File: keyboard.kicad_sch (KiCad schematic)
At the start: 136 parts, among them J1 Conn_01x06_Socket, J2 Conn_01x02_Socket, J3 Conn_01x02_Socket, J4 Conn_01x06_Socket, SW1 SW_Push, SW10 SW_Push, SW11 SW_Push, SW12 SW_Push, SW13 SW_Push, SW14 SW_Push, SW15 SW_Push, SW16 SW_Push, SW17 SW_Push, SW18 SW_Push, SW19 SW_Push, SW2 SW_Push, SW20 SW_Push, SW21 SW_Push, SW22 SW_Push, SW23 SW_Push, SW24 SW_Push, SW25 SW_Push, SW26 SW_Push, SW27 SW_Push, SW28 SW_Push, SW29 SW_Push, SW3 SW_Push, SW30 SW_Push, SW31 SW_Push, SW32 SW_Push, SW33 SW_Push, SW34 SW_Push, SW35 SW_Push, SW36 SW_Push, SW37 SW_Push, SW38 SW_Push, SW39 SW_Push, SW4 SW_Push, SW40 SW_Push, SW41 SW_Push, SW42 SW_Push, SW43 SW_Push, SW44 SW_Push, SW45 SW_Push, SW46 SW_Push, SW47 SW_Push, SW48 SW_Push, SW49 SW_Push, SW5 SW_Push, SW50 SW_Push, SW51 SW_Push, SW52 SW_Push, SW53 SW_Push, SW54 SW_Push, SW55 SW_Push, SW56 SW_Push, SW57 SW_Push, SW58 SW_Push, SW59 SW_Push, SW6 SW_Push, SW60 SW_Push, SW7 SW_Push, SW8 SW_Push, SW9 SW_Push, U1 rp2040-zero, U2 rp2040-zero

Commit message: 実は耐えてた
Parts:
- U1: footprint mcu:rp2040-zero-tht -> mcu:rp2040-zero-smd_reverse_flush_A
- U2: footprint mcu:rp2040-zero-tht -> mcu:rp2040-zero-smd_reverse_flush_B
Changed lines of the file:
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@@
 			)
 		)
-		(property "Footprint" "mcu:rp2040-zero-tht"
+		(property "Footprint" "mcu:rp2040-zero-smd_reverse_flush_A"
 			(at 88.9 48.26 0)
 			(effects
@@
 			)
 		)
-		(property "Footprint" "mcu:rp2040-zero-tht"
+		(property "Footprint" "mcu:rp2040-zero-smd_reverse_flush_B"
 			(at 223.52 48.26 0)
 			(effects

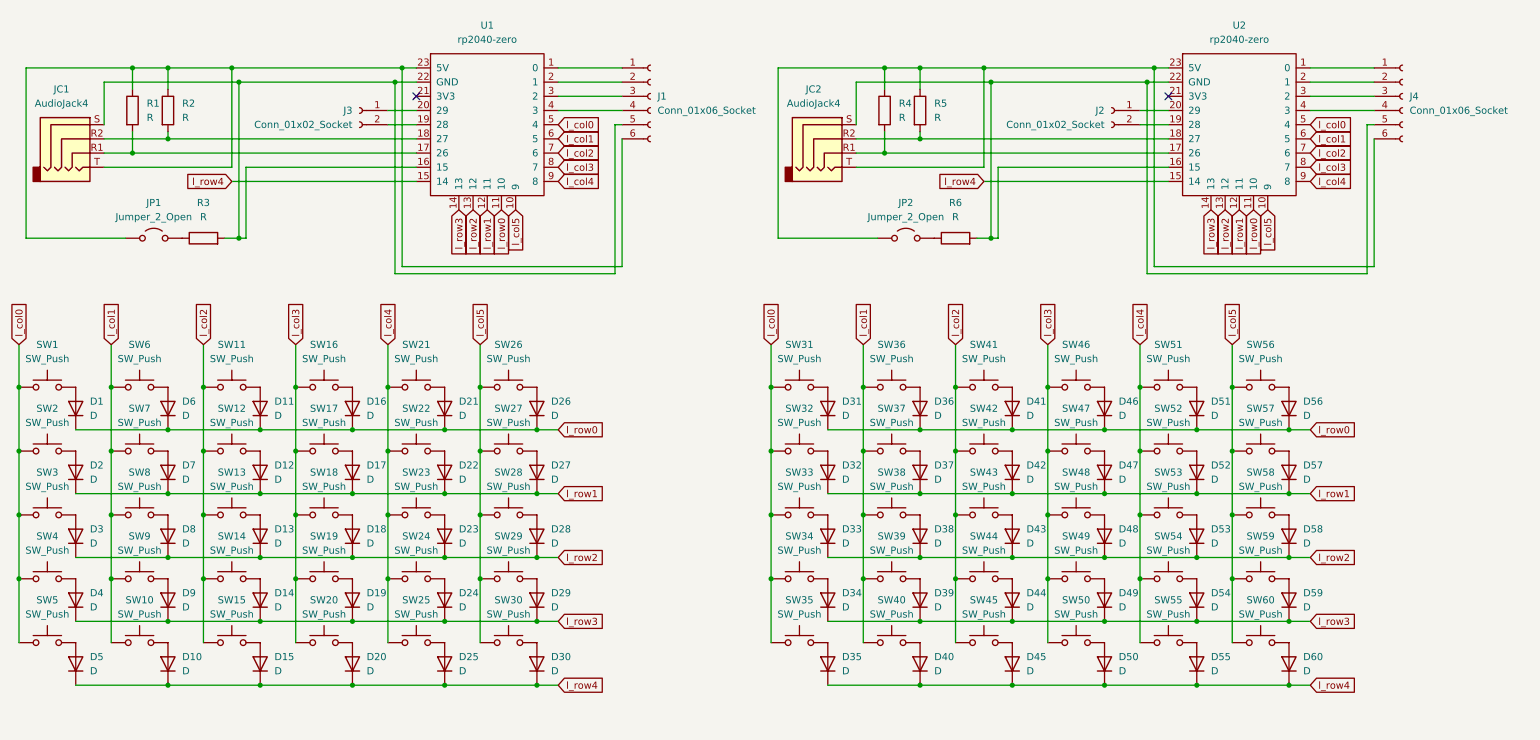
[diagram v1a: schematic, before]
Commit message: 抵抗の配置を直したのでcommit
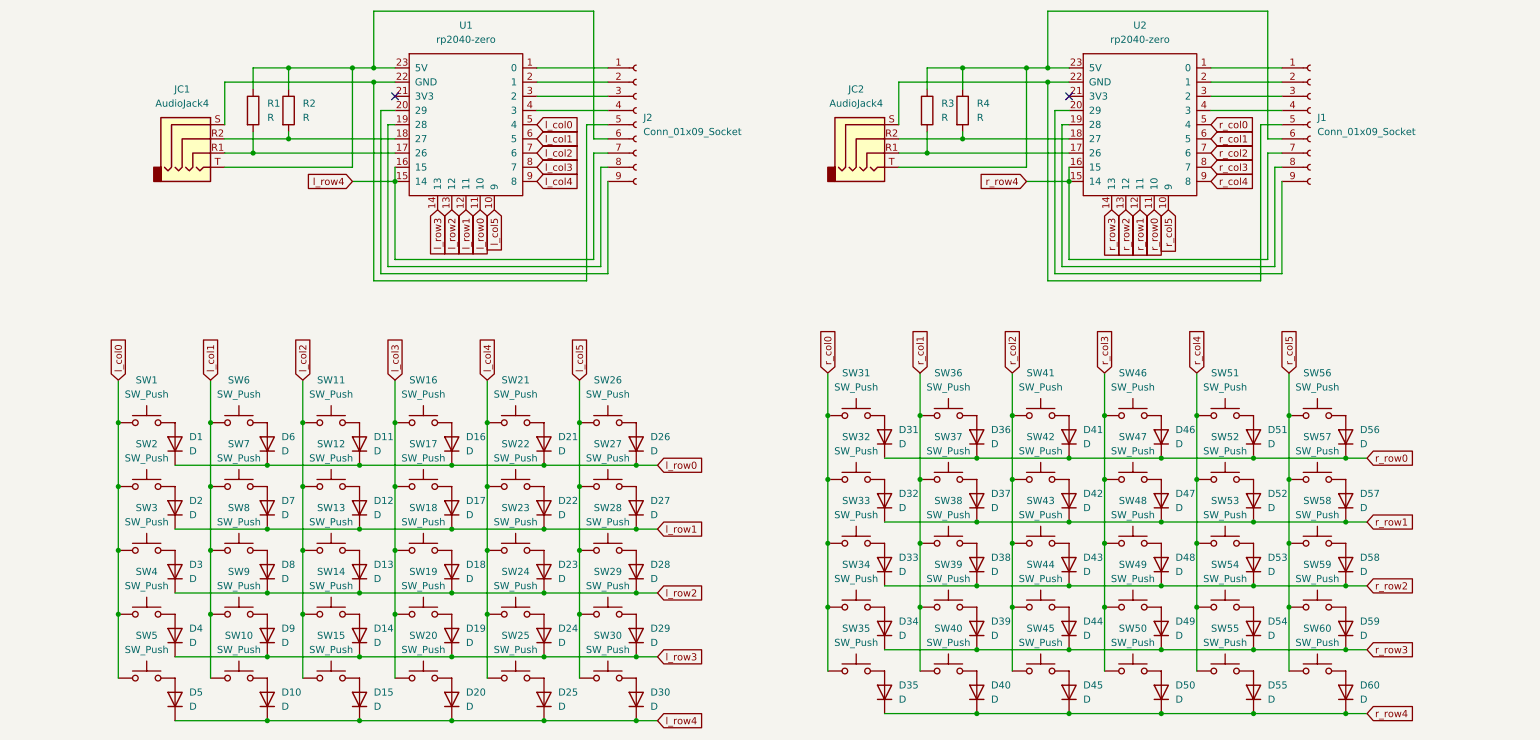
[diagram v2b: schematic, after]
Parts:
- removed J1, J4: Conn_01x06_Socket, Connector_PinHeader_2.54mm:PinHeader_1x06_P2.54mm_Vertical, symbol Connector:Conn_01x06_Socket
- removed J2, J3: Conn_01x02_Socket, Connector_PinHeader_2.54mm:PinHeader_1x02_P2.54mm_Vertical, symbol Connector:Conn_01x02_Socket
- removed JP1, JP2: Jumper_2_Open, Jumper:SolderJumper-2_P1.3mm_Open_Pad1.0x1.5mm, symbol Jumper:Jumper_2_Open
- removed R5, R6: R, Resistor_SMD:R_1206_3216Metric_Pad1.30x1.75mm_HandSolder, symbol Device:R
- added J1, J2: Conn_01x09_Socket, Connector_PinSocket_2.54mm:PinSocket_1x09_P2.54mm_Vertical, symbol Connector:Conn_01x09_Socket
- JC1, JC2: footprint Connector_Audio:Jack_3.5mm_PJ320E_Horizontal -> kbd:MJ-4PP-9
- U1: footprint mcu:rp2040-zero-smd_reverse_flush_A -> mcu:rp2040-zero-smd_flush_front
- U2: footprint mcu:rp2040-zero-smd_reverse_flush_B -> mcu:rp2040-zero-smd_flush_back
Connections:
- net l_col0: no longer SW31.1, SW32.1, SW33.1, SW34.1, SW35.1, U2.5 (4)
- net l_col1: no longer SW36.1, SW37.1, SW38.1, SW39.1, SW40.1, U2.6 (5)
- net l_col2: no longer SW41.1, SW42.1, SW43.1, SW44.1, SW45.1, U2.7 (6)
- net l_col3: no longer SW46.1, SW47.1, SW48.1, SW49.1, SW50.1, U2.8 (7)
- net l_col4: no longer SW51.1, SW52.1, SW53.1, SW54.1, SW55.1, U2.9 (8)
- net l_col5: no longer SW56.1, SW57.1, SW58.1, SW59.1, SW60.1, U2.10 (9)
- net l_row0: no longer D31.1 (K), D36.1 (K), D41.1 (K), D46.1 (K), D51.1 (K), D56.1 (K), U2.11 (10)
- net l_row1: no longer D32.1 (K), D37.1 (K), D42.1 (K), D47.1 (K), D52.1 (K), D57.1 (K), U2.12 (11)
- net l_row2: no longer D33.1 (K), D38.1 (K), D43.1 (K), D48.1 (K), D53.1 (K), D58.1 (K), U2.13 (12)
- net l_row3: no longer D34.1 (K), D39.1 (K), D44.1 (K), D49.1 (K), D54.1 (K), D59.1 (K), U2.14 (13)
- net l_row4: now also U1.16 (15), J2.7 (Pin_7); no longer D35.1 (K), D40.1 (K), D45.1 (K), D50.1 (K), D55.1 (K), D60.1 (K), U2.15 (14)
- net at U1.1 (0): now also J2.1 (Pin_1)
- net at JC1.S, U1.22 (GND): now also J2.5 (Pin_5); no longer R3.2, U1.16 (15)
- net at U1.19 (28): now also J2.8 (Pin_8)
- net at U1.2 (1): now also J2.2 (Pin_2)
- net at U1.20 (29): now also J2.9 (Pin_9)
- net at JC1.T, R1.1, R2.1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: now also J2.6 (Pin_6)
- net at U1.3 (2): now also J2.3 (Pin_3)
- net at U1.4 (3): now also J2.4 (Pin_4)
- net at JC2.S, U2.22 (GND): now also J1.5 (Pin_5); no longer U2.16 (15)
- net at JC2.R1, U2.17 (26): now also R3.2; no longer R4.2
- net at JC2.R2, U2.18 (27): now also R4.2
- net at JC2.T, R4.1, U2.23 (5V): now also R3.1, J1.6 (Pin_6)
- net at U2.1 (0): now also J1.1 (Pin_1)
- net at U2.19 (28): now also J1.8 (Pin_8)
- net at U2.2 (1): now also J1.2 (Pin_2)
- net at U2.20 (29): now also J1.9 (Pin_9)
- net at U2.3 (2): now also J1.3 (Pin_3)
- net at U2.4 (3): now also J1.4 (Pin_4)
- new net r_col0: SW31.1, SW32.1, SW33.1, SW34.1, SW35.1, U2.5 (4)
- new net r_col1: SW36.1, SW37.1, SW38.1, SW39.1, SW40.1, U2.6 (5)
- new net r_col2: SW41.1, SW42.1, SW43.1, SW44.1, SW45.1, U2.7 (6)
- new net r_col3: SW46.1, SW47.1, SW48.1, SW49.1, SW50.1, U2.8 (7)
- new net r_col4: SW51.1, SW52.1, SW53.1, SW54.1, SW55.1, U2.9 (8)
- new net r_col5: SW56.1, SW57.1, SW58.1, SW59.1, SW60.1, U2.10 (9)
- new net r_row0: D31.1 (K), D36.1 (K), D41.1 (K), D46.1 (K), D51.1 (K), D56.1 (K), U2.11 (10)
- new net r_row1: D32.1 (K), D37.1 (K), D42.1 (K), D47.1 (K), D52.1 (K), D57.1 (K), U2.12 (11)
- new net r_row2: D33.1 (K), D38.1 (K), D43.1 (K), D48.1 (K), D53.1 (K), D58.1 (K), U2.13 (12)
- new net r_row3: D34.1 (K), D39.1 (K), D44.1 (K), D49.1 (K), D54.1 (K), D59.1 (K), U2.14 (13)
- new net r_row4: D35.1 (K), D40.1 (K), D45.1 (K), D50.1 (K), D55.1 (K), D60.1 (K), J1.7 (Pin_7), U2.15 (14), U2.16 (15)
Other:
- moved on the sheet: D1, D10, D11, D12, D13, D14, D15, D16, D17, D18, D19, D2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
